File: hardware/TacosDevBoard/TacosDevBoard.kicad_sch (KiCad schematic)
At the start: 6 parts, among them J1 Conn_01x15_Socket, J2 Conn_01x15_Socket, J3 Conn_01x08_Socket, J4 Conn_01x08_Socket

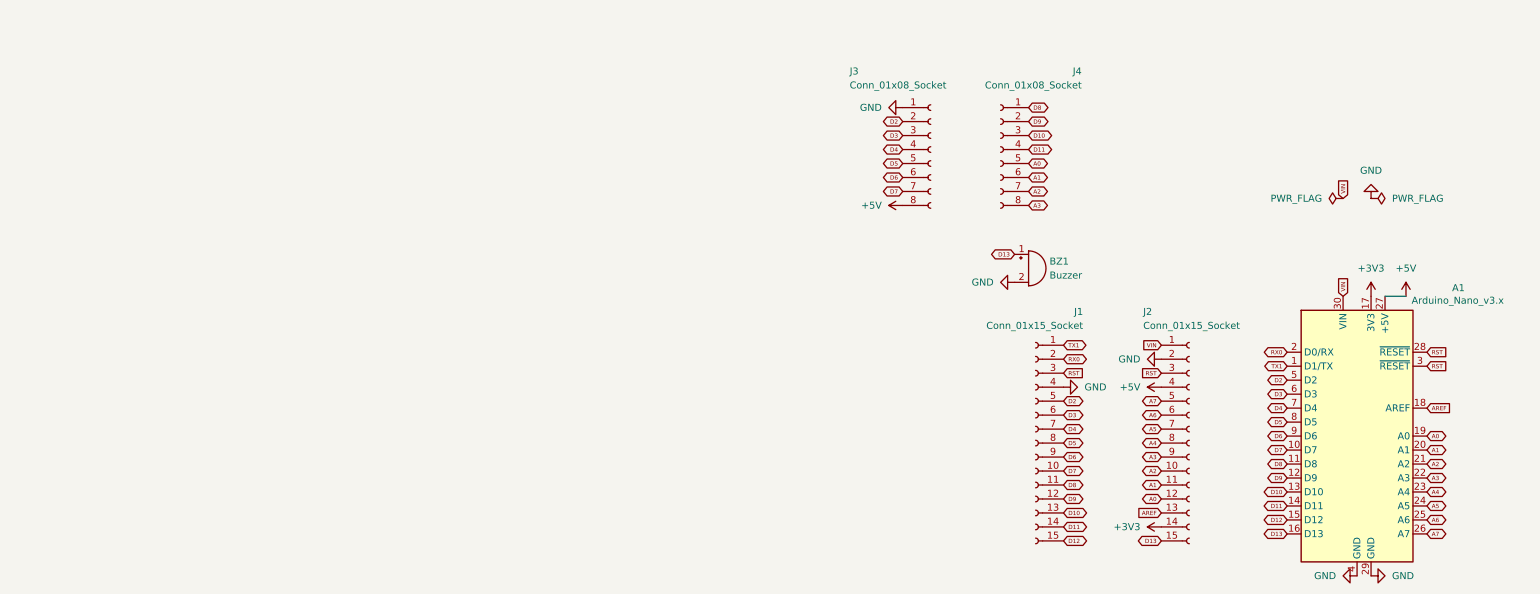
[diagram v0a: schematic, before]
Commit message: finished mega pcb
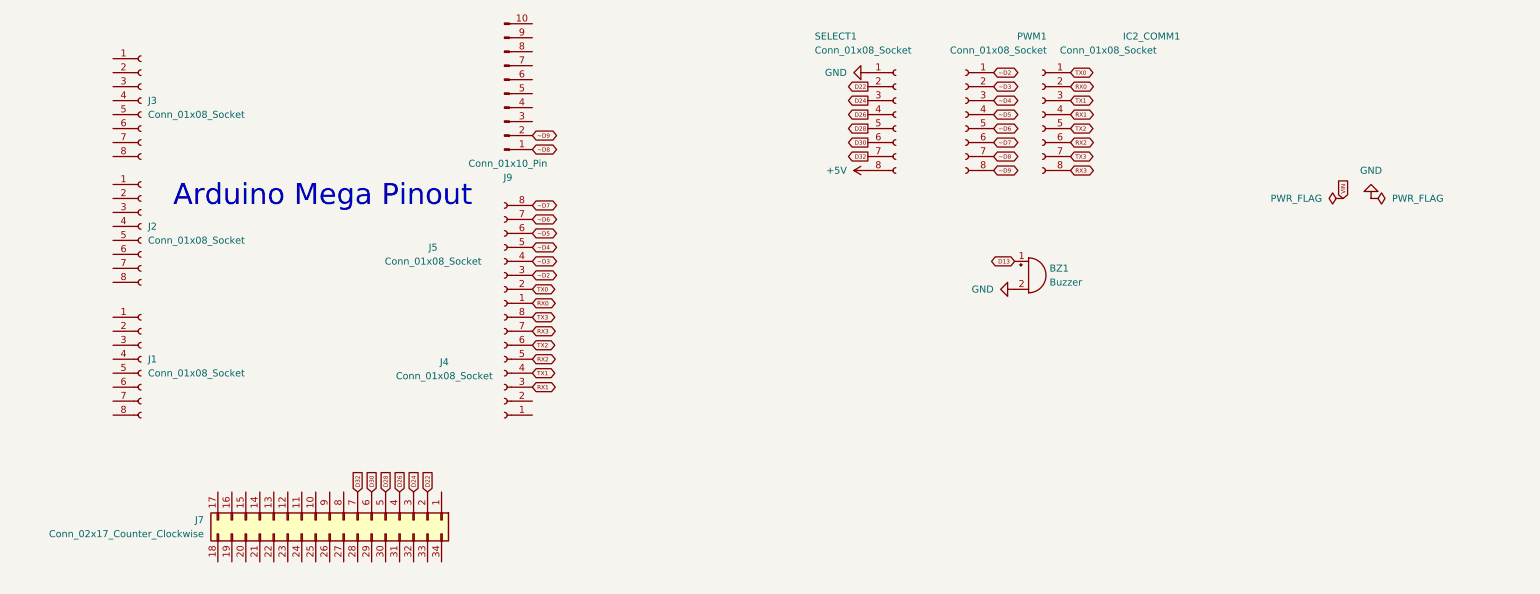
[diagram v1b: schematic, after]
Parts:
- removed A1: Arduino_Nano_v3.x, Module:Arduino_Nano, symbol MCU_Module:Arduino_Nano_v3.x
- removed J1, J2: Conn_01x15_Socket, Connector_PinSocket_2.54mm:PinSocket_1x15_P2.54mm_Vertical, symbol Connector:Conn_01x15_Socket
- added IC2_COMM1: Conn_01x08_Socket, Connector_PinSocket_2.54mm:PinSocket_1x08_P2.54mm_Vertical, symbol Connector:Conn_01x08_Socket
- added J1, J2, J3, J4, J5: Conn_01x08_Socket, Connector_PinHeader_2.54mm:PinHeader_1x08_P2.54mm_Vertical, symbol Connector:Conn_01x08_Socket
- added J7: Conn_02x17_Counter_Clockwise, Connector_PinHeader_2.54mm:PinHeader_2x17_P2.54mm_Vertical, symbol Connector_Generic:Conn_02x17_Counter_Clockwise
- added J9: Conn_01x10_Pin, Connector_PinHeader_2.54mm:PinHeader_1x10_P2.54mm_Vertical, symbol Connector:Conn_01x10_Pin
- renumbered J4 to PWM1, J3 to SELECT1
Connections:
- net RX0: now also IC2_COMM1.2 (Pin_2), J5.1 (Pin_1)
- net TX1: now also IC2_COMM1.3 (Pin_3), J4.4 (Pin_4)
- net A0 renamed ~D6
- net ~D6: now also J5.7 (Pin_7)
- net A1 renamed ~D7
- net ~D7: now also J5.8 (Pin_8)
- net A2 renamed ~D8
- net ~D8: now also J9.1 (Pin_1)
- net A3 renamed ~D9
- net ~D9: now also J9.2 (Pin_2)
- net D10 renamed ~D4
- net ~D4: now also J5.5 (Pin_5)
- net D11 renamed ~D5
- net ~D5: now also J5.6 (Pin_6)
- net D2 renamed D22
- net D22: now also J7.2 (Pin_2)
- net D3 renamed D24
- net D24: now also J7.3 (Pin_3)
- net D4 renamed D26
- net D26: now also J7.4 (Pin_4)
- net D5 renamed D28
- net D28: now also J7.5 (Pin_5)
- net D6 renamed D30
- net D30: now also J7.6 (Pin_6)
- net D7 renamed D32
- net D32: now also J7.7 (Pin_7)
- net D8 renamed ~D2
- net ~D2: now also J5.3 (Pin_3)
- net D9 renamed ~D3
- net ~D3: now also J5.4 (Pin_4)
- new net RX1: IC2_COMM1.4 (Pin_4), J4.3 (Pin_3)
- new net RX2: IC2_COMM1.6 (Pin_6), J4.5 (Pin_5)
- new net RX3: IC2_COMM1.8 (Pin_8), J4.7 (Pin_7)
- new net TX0: IC2_COMM1.1 (Pin_1), J5.2 (Pin_2)
- new net TX2: IC2_COMM1.5 (Pin_5), J4.6 (Pin_6)
- new net TX3: IC2_COMM1.7 (Pin_7), J4.8 (Pin_8)
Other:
- note added: "Arduino Mega Pinout"
- moved on the sheet: BZ1, PWM1, SELECT1
